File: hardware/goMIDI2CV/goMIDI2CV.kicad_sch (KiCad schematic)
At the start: 15 parts, among them U1 ATtiny85-20P, U2 LM324

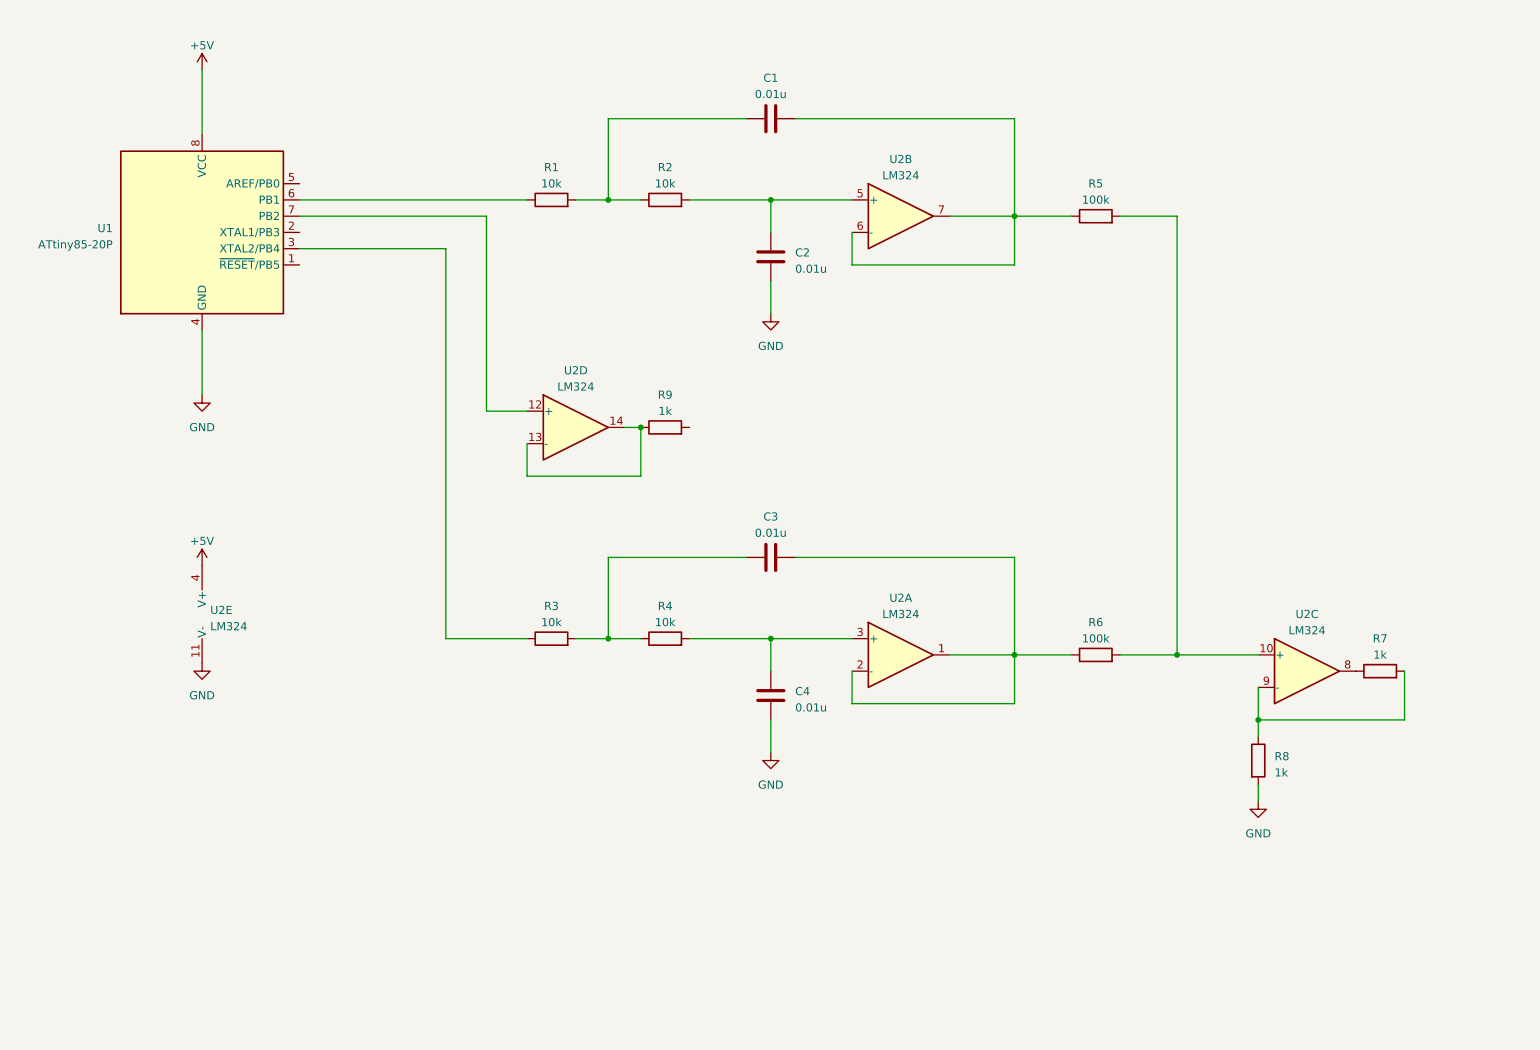
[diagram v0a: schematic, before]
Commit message: updated schematic
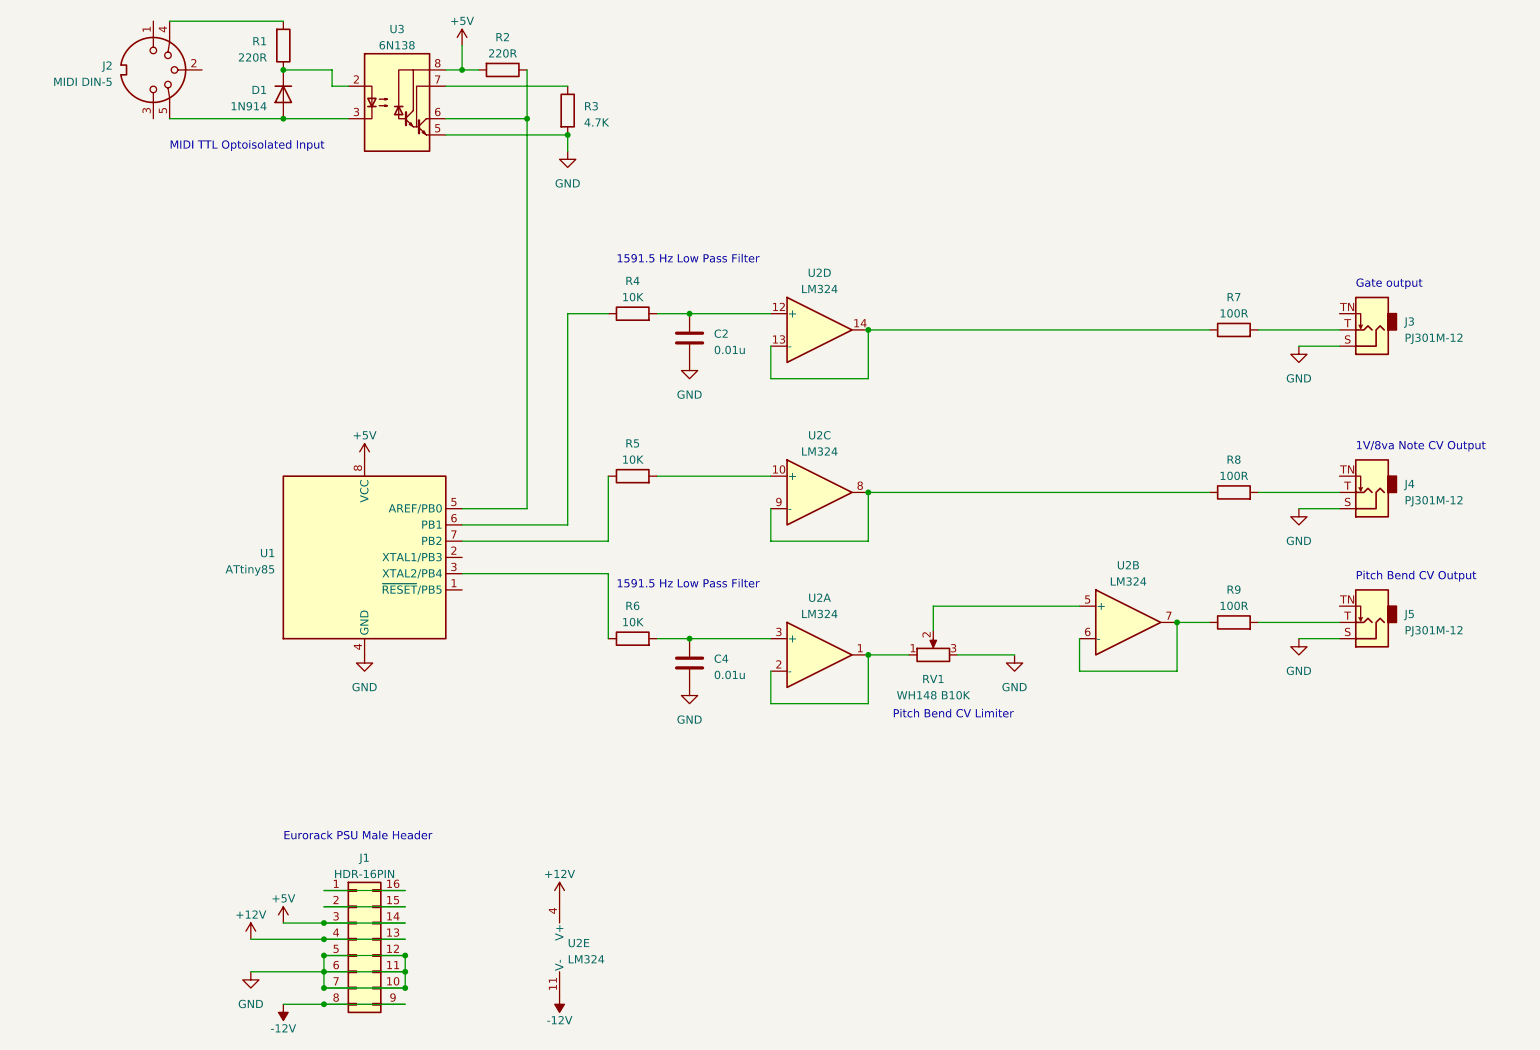
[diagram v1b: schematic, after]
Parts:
- removed C1, C3: 0.01u, Capacitor_THT:C_Disc_D5.0mm_W2.5mm_P2.50mm, symbol Device:C
- removed R5, R6: 100k, Resistor_THT:R_Axial_DIN0207_L6.3mm_D2.5mm_P5.08mm_Vertical, symbol Device:R
- added D1: 1N914, Diode_THT:D_DO-35_SOD27_P7.62mm_Horizontal, symbol Diode:1N914
- added J1: HDR-16PIN, symbol Connector_Generic:Conn_02x08_Counter_Clockwise
- added J2: MIDI DIN-5, symbol Connector:DIN-5_180degree
- added J3, J4, J5: PJ301M-12, symbol Connector_Audio:AudioJack2_SwitchT
- added R2: 220R, Resistor_THT:R_Axial_DIN0207_L6.3mm_D2.5mm_P5.08mm_Vertical, symbol Device:R
- added R9: 100R, Resistor_THT:R_Axial_DIN0207_L6.3mm_D2.5mm_P5.08mm_Vertical, symbol Device:R
- added RV1: WH148 B10K, symbol Device:R_Potentiometer
- added U3: 6N138, symbol Isolator:6N138
- R1: value 10k -> 220R
- R3: value 10k -> 4.7K
- R4: renamed from R2; value 10k -> 10K
- R5: renamed from R9; value 1k -> 10K
- R6: renamed from R4; value 10k -> 10K
- R7, R8: value 1k -> 100R
- U1: value ATtiny85-20P -> ATtiny85
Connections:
- net +5V: now also J1.14 (Pin_14), J1.3 (Pin_3), R2.2, U3.8 (VCC); no longer U2.4 (V+)
- net GND: now also R3.2, J1.10 (Pin_10), J1.11 (Pin_11), J1.12 (Pin_12), J1.5 (Pin_5), J1.6 (Pin_6), J1.7 (Pin_7), J3.S, J4.S, J5.S, RV1.3, U3.5 (GND); no longer R8.2, U2.11 (V-)
- net at U2.6 (-), U2.7: now also R9.1
- net at R1.2: now also J2.4; no longer R4.1
- net at U2.10 (+): now also R5.2
- net at U2.1, U2.2 (-): now also RV1.1
- net at R6.1: now also U1.3 (XTAL2/PB4); no longer R3.2
- net at R8.1, U2.9 (-): now also U2.8; no longer R7.2
- net at U2.12 (+): now also C2.2, R4.2; no longer U1.7 (PB2)
- net at U2.13 (-), U2.14: now also R7.1; no longer R5.1
- net at R3.1: now also U3.7 (VO1); no longer U1.3 (XTAL2/PB4)
- net at U1.5 (AREF/PB0): now also R2.1, U3.6 (VO2)
- net at R1.1: now also D1.1 (K), U3.2 (C1); no longer U1.6 (PB1)
- new net: D1.2 (A), J2.5, U3.3 (C2)
- new net: RV1.2, U2.5 (+)
- new net: J3.T, R7.2
- new net: J4.T, R8.2
- new net: J5.T, R9.2
- new net: R4.1, U1.6 (PB1)
- new net: R5.1, U1.7 (PB2)
- new net: J1.1 (Pin_1), J1.16 (Pin_16)
- new net: J1.15 (Pin_15), J1.2 (Pin_2)
- new net +12V: J1.13 (Pin_13), J1.4 (Pin_4), U2.4 (V+)
- new net -12V: J1.8 (Pin_8), J1.9 (Pin_9), U2.11 (V-)
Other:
- note added: "1591.5 Hz Low Pass Filter"
- note added: "1V/8va Note CV Output"
- note added: "Eurorack PSU Male Header"
- note added: "Gate output"
- note added: "MIDI TTL Optoisolated Input"
- note added: "Pitch Bend CV Limiter"
- note added: "Pitch Bend CV Output"
- company: (none) -> Aether Soundlab
- title: (none) -> goMIDI2CV
- moved on the sheet: C2, C4, R4, R5, R6, U1, U2A, U2B, U2C, U2D, U2E
